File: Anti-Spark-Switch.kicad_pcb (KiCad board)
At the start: 2 copper layers, 16 parts, among them P1 Pad_Conn, P2 Pad_Conn, P3 Screw_Terminal, P4 Screw_Terminal, P5 Pad_Conn, P6 Pad_Conn, P7 CONN_01X02, Q1 IRFS7530, Q2 IRFS7530, Q3 IRFS7530, SW1 SW_PUSH

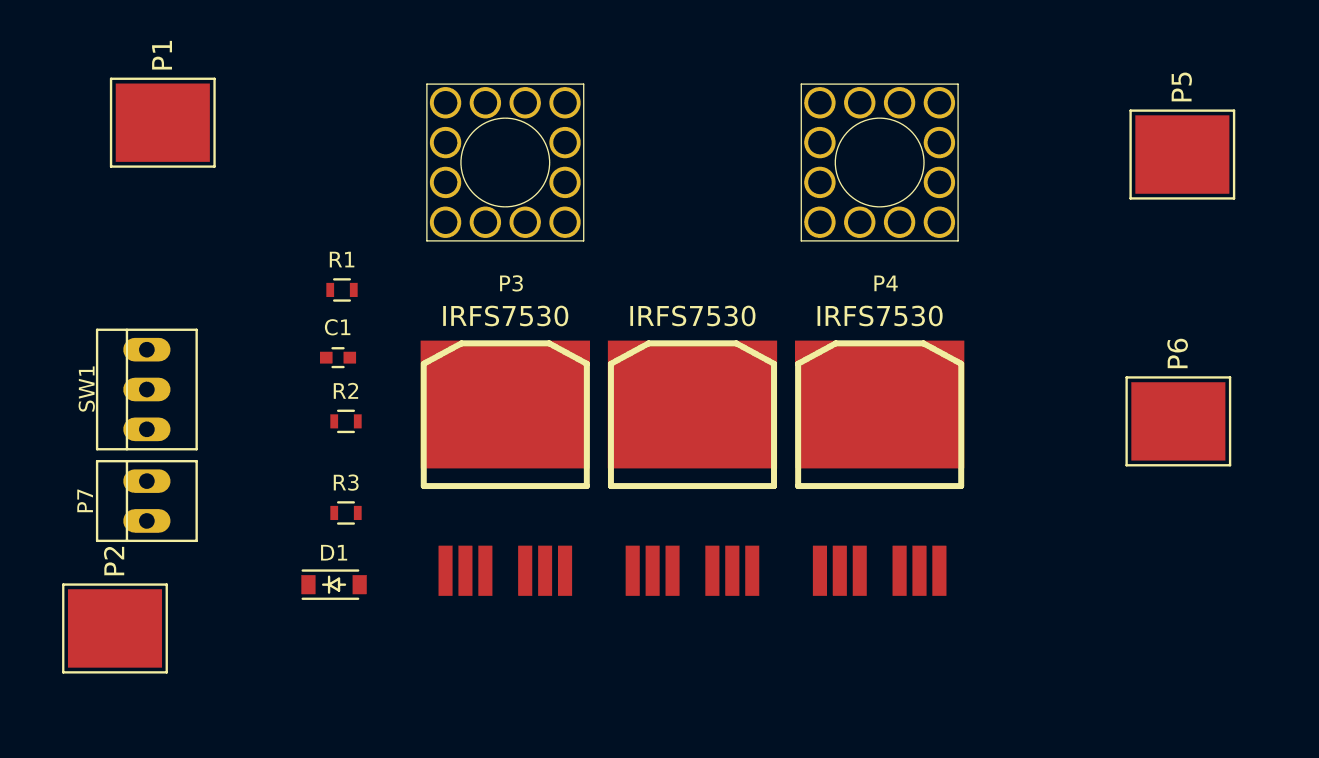
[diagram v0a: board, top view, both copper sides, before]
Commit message: continued work on PCB
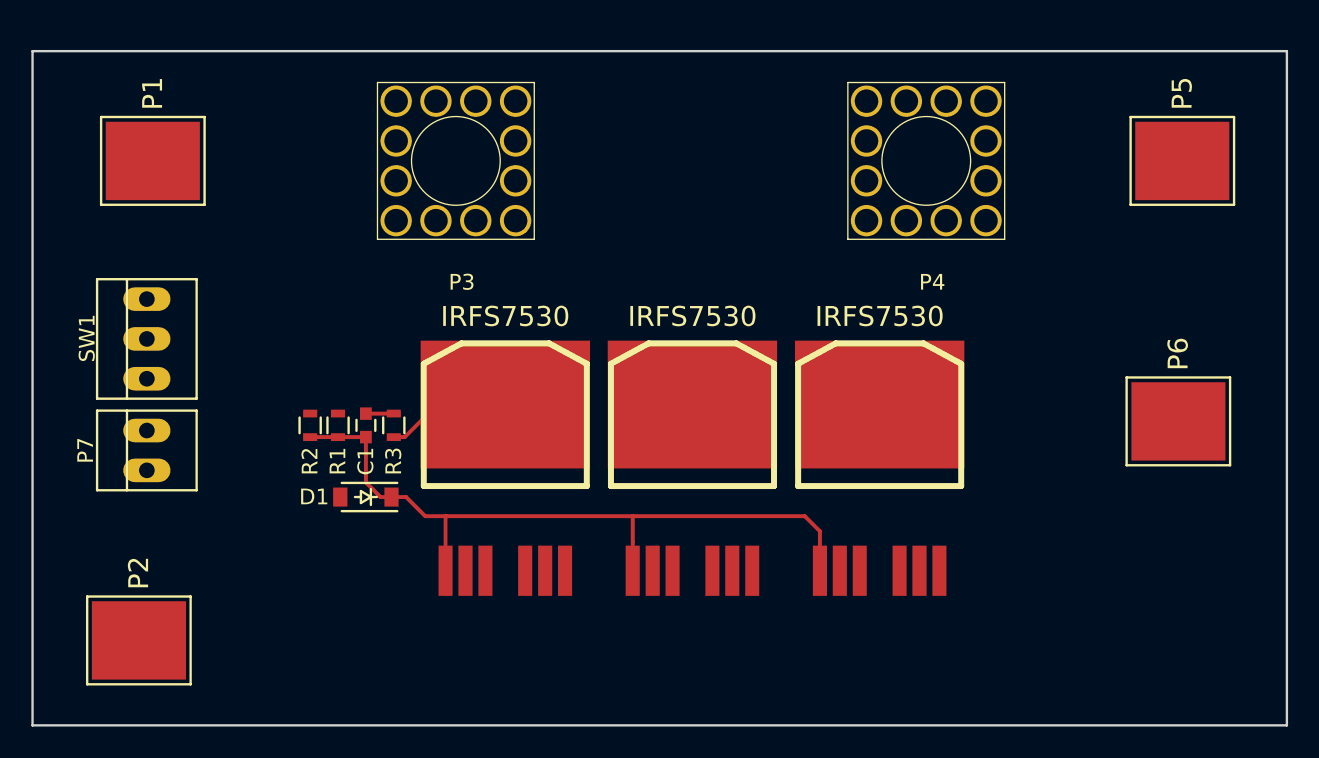
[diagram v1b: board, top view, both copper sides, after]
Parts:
- moved R1 8.64 mm to (189.5, 70.9), turned to 270 degrees
- moved R3 6.37 mm to (193.0, 70.9), turned to 90 degrees
- moved D1 5.95 mm to (191.3, 75.4), turned to 180 degrees
- moved C1 4.67 mm to (191.3, 70.9), turned to 270 degrees
- moved P7 3.23 mm to (177.3, 72.5)
- moved SW1 3.23 mm to (177.3, 65.4)
- moved P3 3.15 mm to (197.0, 54.0)
- moved P4 2.97 mm to (227.0, 54.0)
- moved P1 2.52 mm to (177.7, 54.0)
- moved R2 2.30 mm to (187.7, 70.9), turned to 90 degrees
- moved P2 1.70 mm to (176.8, 84.6)
- moved P5 0.41 mm to (243.3, 54.0)
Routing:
- net Net-(C1-Pad2): track 0.00 -> 46.2 mm
- net Net-(P6-Pad1): track 0.00 -> 7.97 mm
- net Net-(C1-Pad1): track 0.00 -> 1.78 mm
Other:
- board outline added: 80 x 43 mm
